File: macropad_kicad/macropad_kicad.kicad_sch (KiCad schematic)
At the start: 26 parts, among them J1 OLED_128x64, SW1 RotaryEncoder_Switch, U1 MOUDLE-SEEEDUINO-XIAO

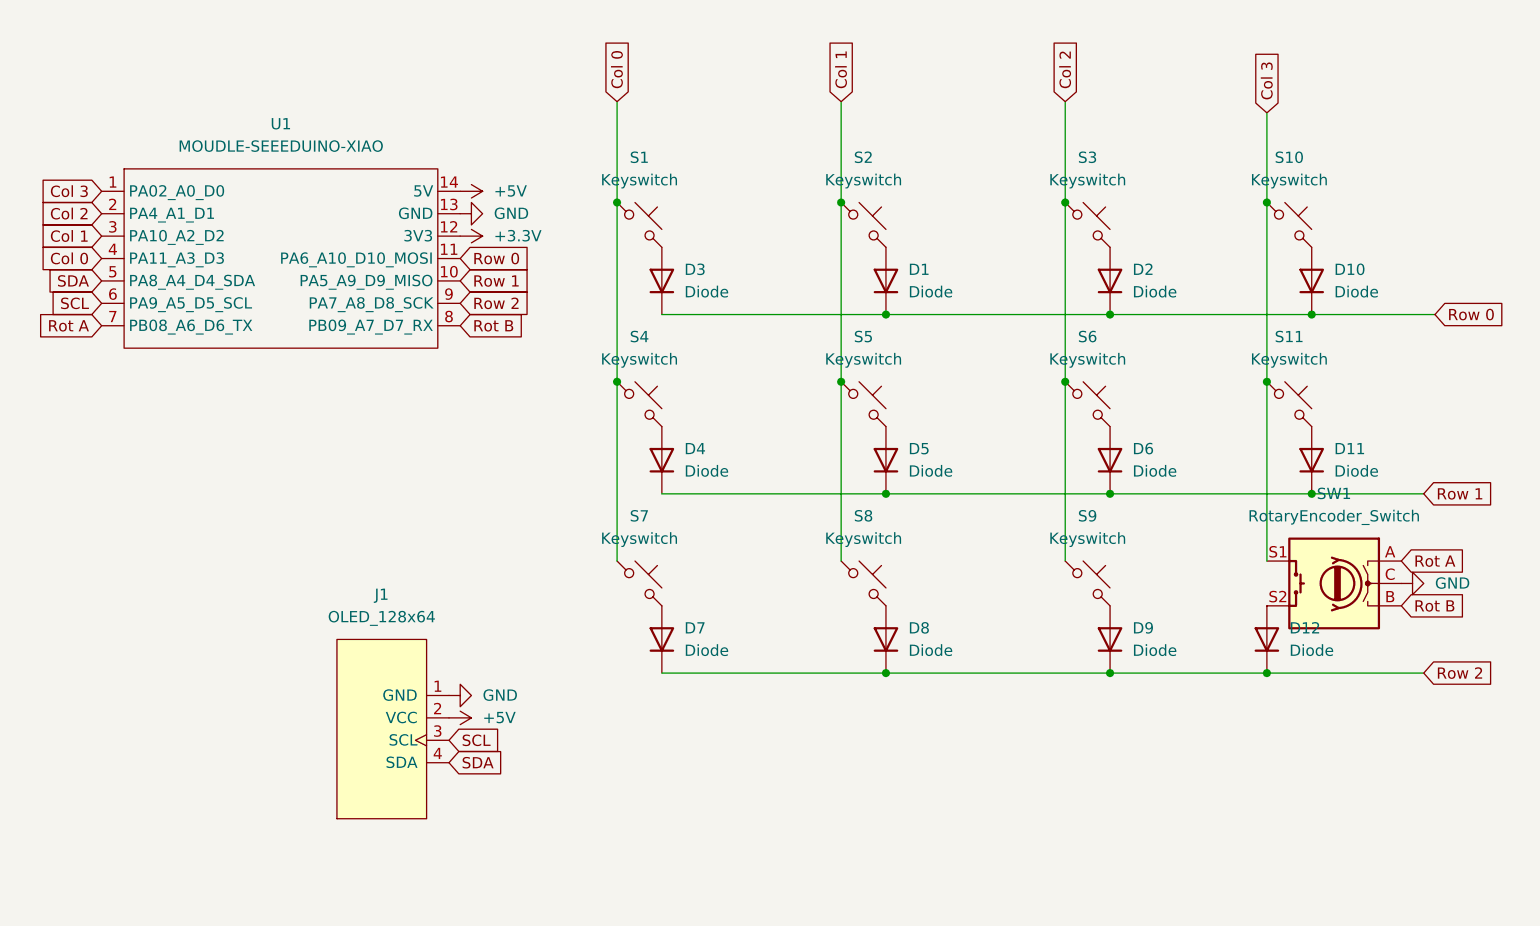
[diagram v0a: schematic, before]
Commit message: fixed scheme
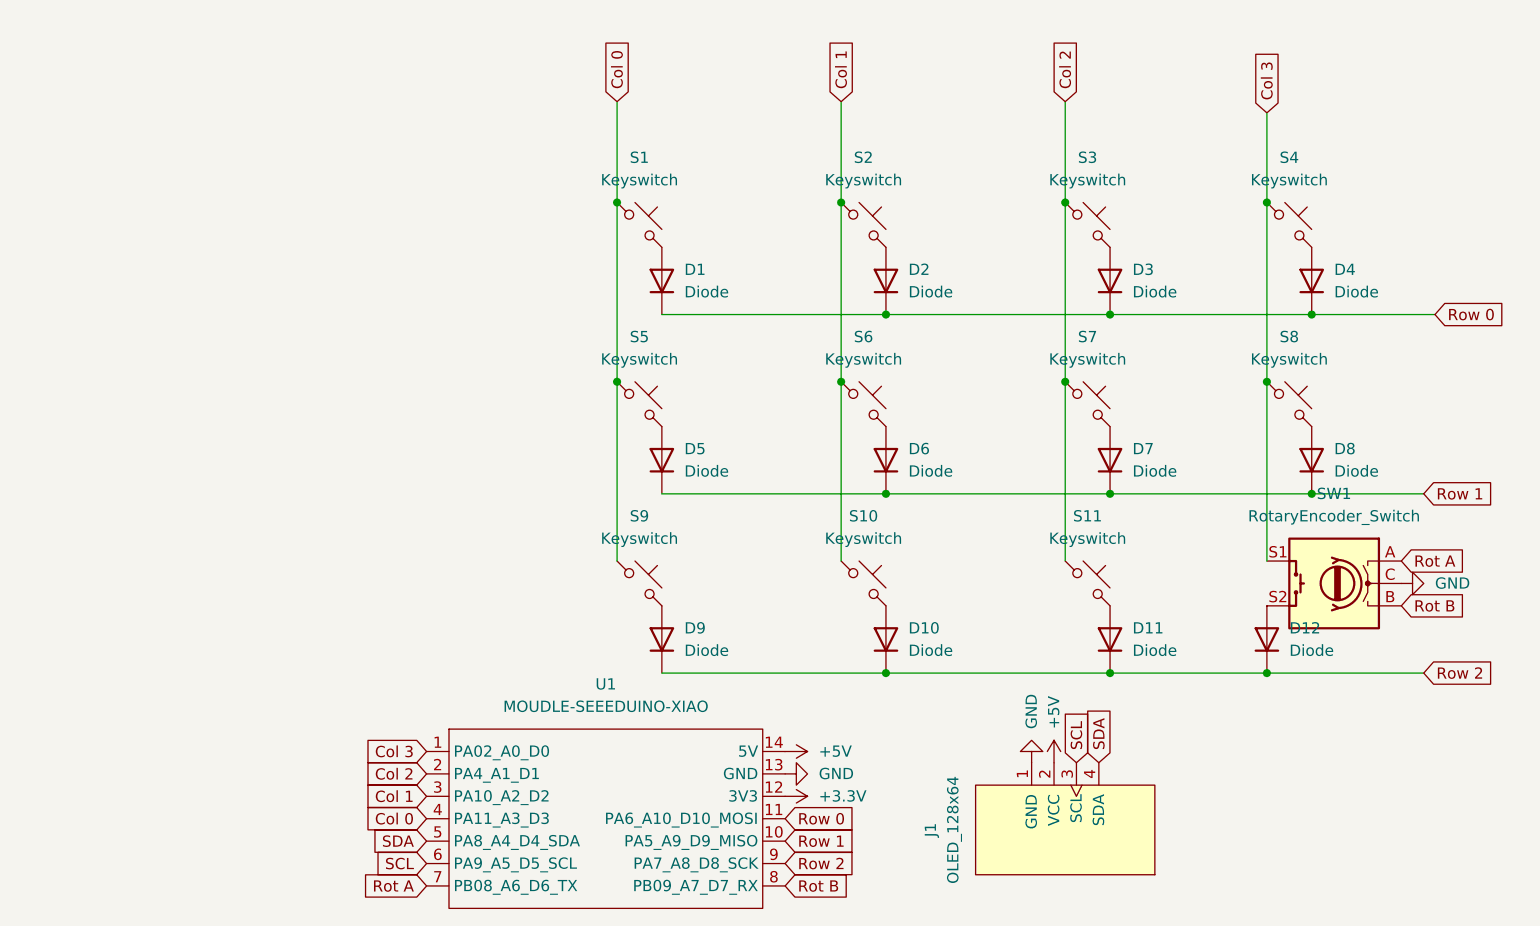
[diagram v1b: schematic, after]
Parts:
- S1, S10, S11, S2, S3, S4, S5, S6, S7, S8, S9: footprint Button_Switch_Keyboard:SW_Cherry_MX_1.00u_PCB -> ScottoKeebs_MX:MX_PCB_1.00u
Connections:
- net Col 0: now also S5.1, S9.1; no longer S4.1, S7.1
- net Col 1: now also S10.1, S6.1; no longer S5.1, S8.1
- net Col 2: now also S11.1, S7.1; no longer S6.1, S9.1
- net Col 3: now also S4.1, S8.1; no longer S10.1, S11.1
- net Row 0: now also D4.1 (K); no longer D10.1 (K)
- net Row 1: now also D7.1 (K), D8.1 (K); no longer D11.1 (K), D4.1 (K)
- net Row 2: now also D10.1 (K), D11.1 (K); no longer D7.1 (K), D8.1 (K)
- net at D2.2 (A): now also S2.2; no longer S3.2
- net at D1.2 (A): now also S1.2; no longer S2.2
- net at D3.2 (A): now also S3.2; no longer S1.2
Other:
- moved on the sheet: D1, D10, D11, D2, D3, D4, D5, D6, D7, D8, D9, J1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
